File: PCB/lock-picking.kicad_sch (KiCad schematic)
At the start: 12 parts, among them CN1 B2B-XH-A, CN2 B2B-XH-A, CN3 B2B-XH-A, U1 ESP32-C3-SuperMini, U2 DRV8876PWPR, U3 MLX90393SLW-ABA-011-RE, U4 B4B-XH-A, U5 B4B-XH-A

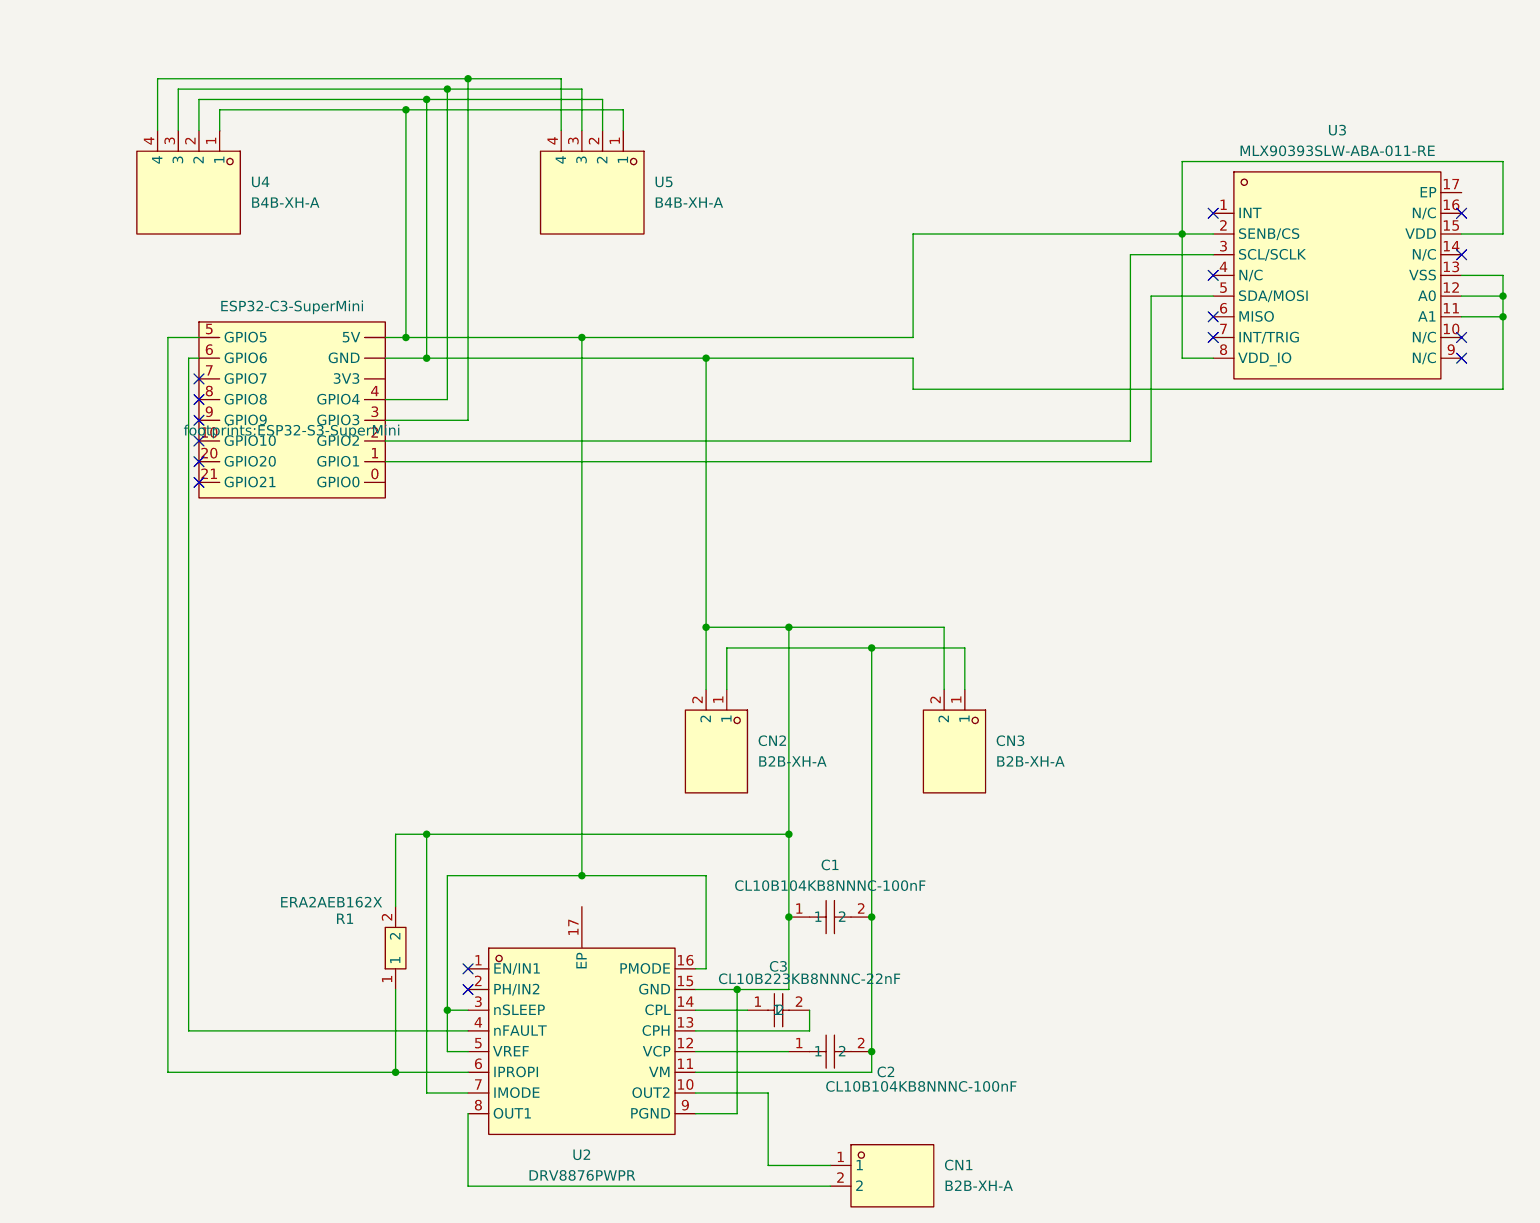
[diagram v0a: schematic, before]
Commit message: kicad
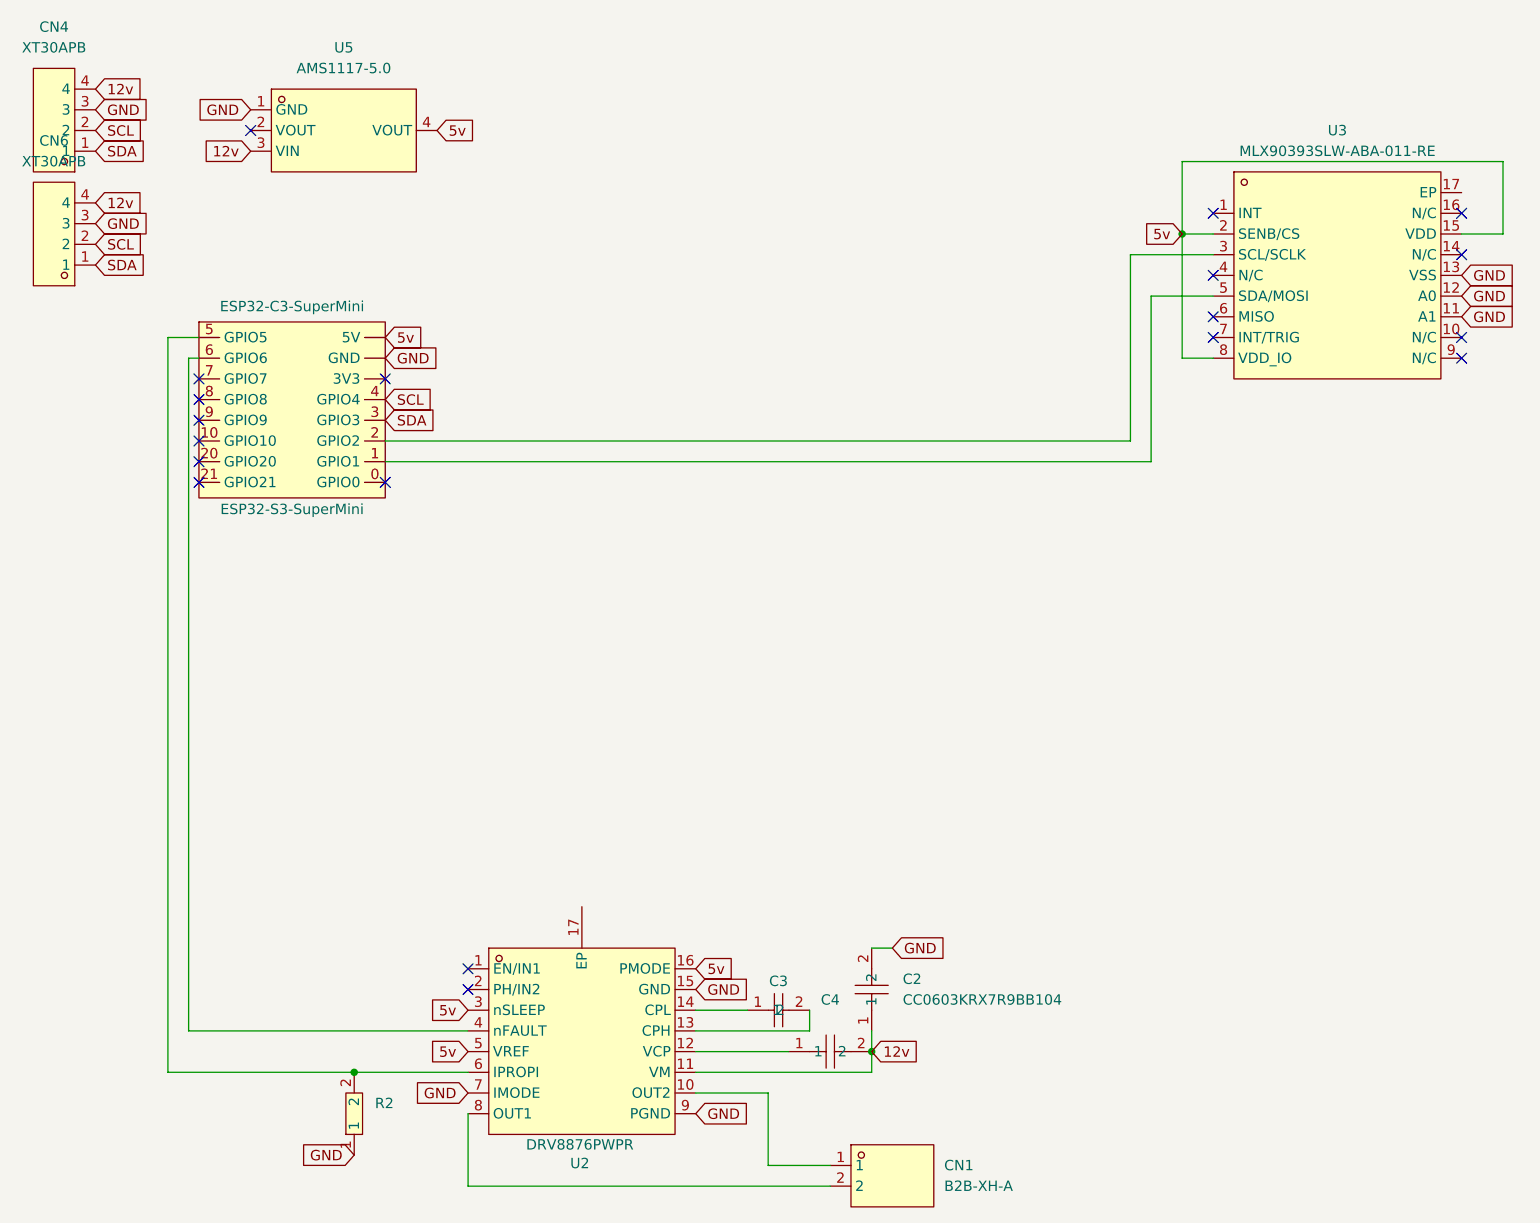
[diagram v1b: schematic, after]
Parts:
- removed C1, C2: CL10B104KB8NNNC-100nF, EasyEDA:C0603, symbol EasyEDA:CL10B104KB8NNNC
- removed CN2, CN3: B2B-XH-A, EasyEDA:CONN-TH_B2B-XH-A-LF-SN, symbol EasyEDA:B2B-XH-A
- removed R1: ERA2AEB162X, EasyEDA:R0402, symbol EasyEDA:ERA2AEB162X
- removed U4, U5: B4B-XH-A, EasyEDA:CONN-TH_B4B-XH-A-LF-SN, symbol EasyEDA:B4B-XH-A
- added C2, C4: CC0603KRX7R9BB104, EasyEDA:C0603, symbol EasyEDA:CC0603KRX7R9BB104
- added CN4, CN6: XT30APB, EasyEDA:CONN-TH_XT30APB, symbol EasyEDA:XT30APB
- added R2: 0603WAF1501T5E, EasyEDA:R0603, symbol EasyEDA:0603WAF1501T5E
- added U5: AMS1117-5.0, EasyEDA:SOT-223_L6.5-W3.5-P2.30-LS7.0-BR, symbol EasyEDA:AMS1117-5.0
- U1: footprint footprints:ESP32-S3-SuperMini -> ESP32-S3-SuperMini
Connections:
- net 5v: now reaches U1. (3V3), U2.16 (PMODE), U2.3 (nSLEEP), U2.5 (VREF), U3.15 (VDD), U3.2 (SENB/CS), U3.8 (VDD_IO)
- net 5v: now also U5.4 (VOUT)
- net GND: now reaches U1. (3V3), U2.15 (GND), U2.7 (IMODE), U2.9 (PGND), U3.11 (A1), U3.12 (A0), U3.13 (VSS)
- net GND: now also C2.2, CN4.3, CN6.3, R2.1, U5.1 (GND)
- net SCL: now reaches U1.4 (GPIO4)
- net SCL: now also CN4.2, CN6.2
- net SDA: now reaches U1.3 (GPIO3)
- net SDA: now also CN4.1, CN6.1
- net 12v: now reaches U2.11 (VM)
- net 12v: now also C2.1, C4.2, CN4.4, CN6.4, U5.3 (VIN)
- net at U1.5 (GPIO5), U2.6 (IPROPI): now also R2.2
- net at U2.12 (VCP): now also C4.1
- no-connect marks 16 -> 19
